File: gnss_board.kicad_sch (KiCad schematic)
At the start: 67 parts, among them J1 Conn_01x10_Pin, T1 LMUN2211LT1G(SOT-23), U1 H1102NL, U2 LAN8710A, U3 TPS2375D, U4 TX4138(ESOIC-8)

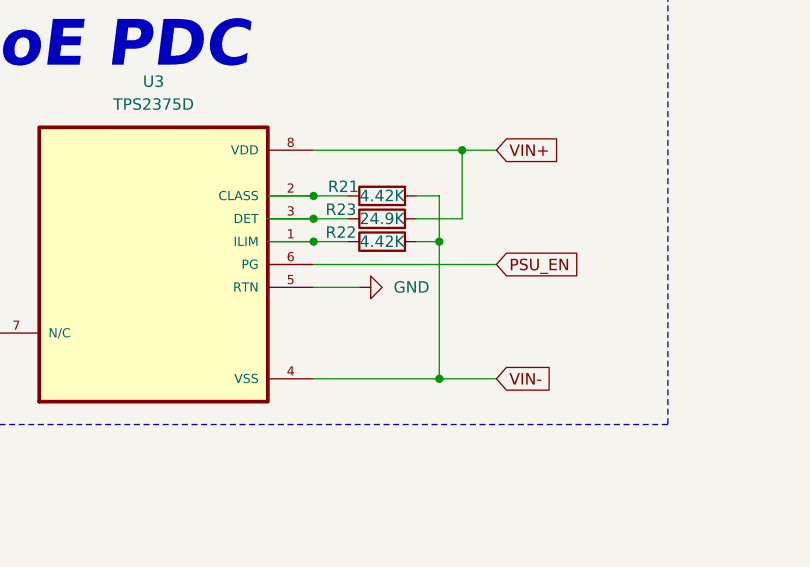
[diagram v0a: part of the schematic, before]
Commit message: Slowly grinding
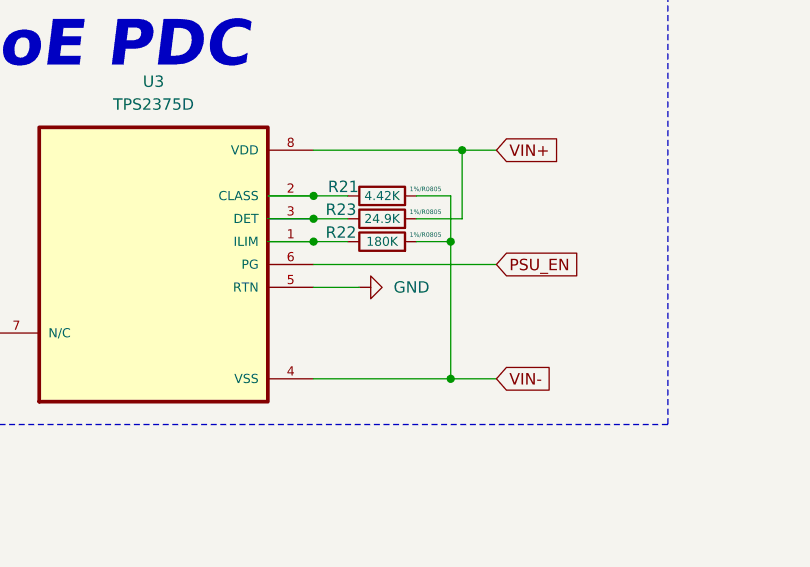
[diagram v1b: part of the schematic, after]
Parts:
- R21: footprint (none) -> Resistor_SMD:R_0805_2012Metric; Info (none) -> 1%/R0805
- R22: value 4.42K -> 180K; footprint (none) -> Resistor_SMD:R_0805_2012Metric; Info (none) -> 1%/R0805
- R23: Info (none) -> 1%/R0805
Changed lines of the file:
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@@
 	)
 	(junction
-		(at 69.85 130.81)
-		(diameter 0)
-		(color 0 0 0 0)
-	)
-	(junction
 		(at 100.33 33.02)
 		(diameter 0)
@@
 	)
 	(junction
+		(at 71.12 130.81)
+		(diameter 0)
+		(color 0 0 0 0)
+	)
+	(junction
+		(at 71.12 146.05)
+		(diameter 0)
+		(color 0 0 0 0)
+	)
+	(junction
 		(at 335.28 30.48)
 		(diameter 0)
@@
 	)
 	(junction
-		(at 69.85 146.05)
-		(diameter 0)
-		(color 0 0 0 0)
-	)
-	(junction
 		(at 257.81 45.72)
 		(diameter 0)
@@
 	(wire
 		(pts
-			(xy 55.88 146.05) (xy 69.85 146.05)
+			(xy 55.88 146.05) (xy 71.12 146.05)
 		)
 		(stroke
@@
 	(wire
 		(pts
-			(xy 67.31 125.73) (xy 69.85 125.73)
+			(xy 67.31 125.73) (xy 71.12 125.73)
 		)
 		(stroke
@@
 	(wire
 		(pts
-			(xy 69.85 125.73) (xy 69.85 130.81)
+			(xy 71.12 125.73) (xy 71.12 130.81)
 		)
 		(stroke
@@
 	(wire
 		(pts
-			(xy 69.85 130.81) (xy 69.85 146.05)
+			(xy 71.12 130.81) (xy 71.12 146.05)
 		)
 		(stroke
@@
 	(wire
 		(pts
-			(xy 69.85 146.05) (xy 76.2 146.05)
-		)
-		(stroke
-			(width 0)
-			(type default)
-		)
-	)
-	(wire
-		(pts
 			(xy 48.26 43.18) (xy 53.34 43.18)
 		)
@@
 	(wire
 		(pts
-			(xy 67.31 130.81) (xy 69.85 130.81)
+			(xy 67.31 130.81) (xy 71.12 130.81)
 		)
 		(stroke
@@
 	(wire
 		(pts
+			(xy 71.12 146.05) (xy 76.2 146.05)
+		)
+		(stroke
+			(width 0)
+			(type default)
+		)
+	)
+	(wire
+		(pts
 			(xy 54.61 59.69) (xy 54.61 54.61)
 		)
@@
 			(effects
 				(font
-					(size 1.27 1.27)
+					(size 1 1)
 				)
 			)
 		)
-		(property "Footprint" ""
+		(property "Footprint" "Resistor_SMD:R_0805_2012Metric"
 			(at 63.5 127.508 90)
 			(effects
@@
 			)
 		)
+		(property "Info" "1%/R0805"
+			(at 68.326 124.968 90)
+			(effects
+				(font
+					(size 0.5 0.5)
+				)
+			)
+		)
 		(pin "2"
 		)
@@
 			)
 		)
-		(property "Value" "4.42K"
+		(property "Value" "180K"
 			(at 63.5 130.81 90)
 			(effects
 				(font
-					(size 1.27 1.27)
+					(size 1 1)
 				)
 			)
 		)
-		(property "Footprint" ""
+		(property "Footprint" "Resistor_SMD:R_0805_2012Metric"
 			(at 63.5 132.588 90)
 			(effects
@@
 			)
 		)
+		(property "Info" "1%/R0805"
+			(at 68.326 130.048 90)
+			(effects
+				(font
+					(size 0.5 0.5)
+				)
+			)
+		)
 		(pin "2"
 		)
@@
 			(effects
 				(font
-					(size 1.27 1.27)
+					(size 1 1)
 				)
 			)
@@
 			)
 		)
+		(property "Info" "1%/R0805"
+			(at 68.326 127.508 90)
+			(effects
+				(font
+					(size 0.5 0.5)
+				)
+			)
+		)
